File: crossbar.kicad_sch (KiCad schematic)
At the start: 6 parts

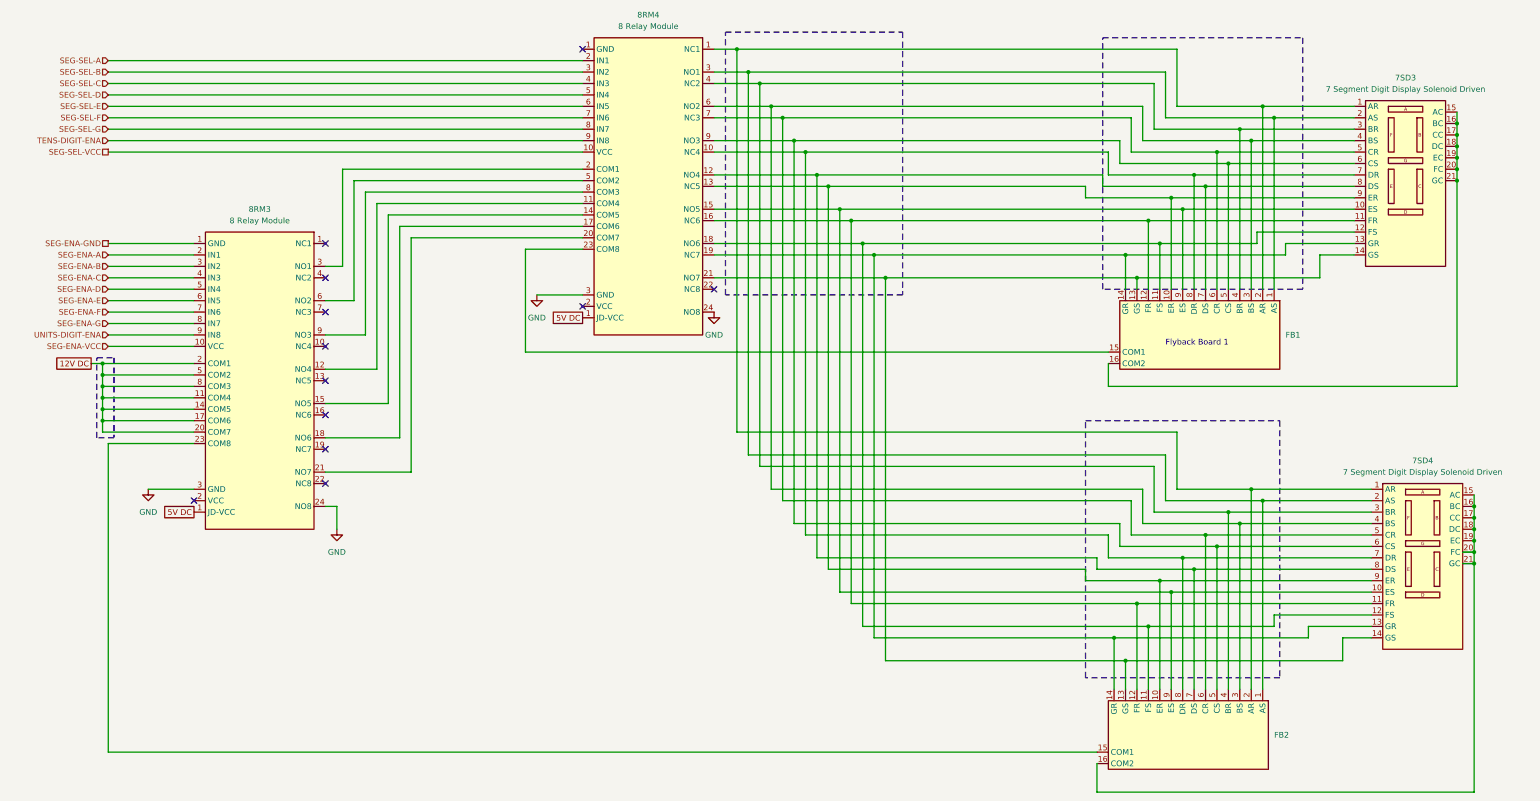
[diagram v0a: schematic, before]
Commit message: lots of diagram changes and software dir.
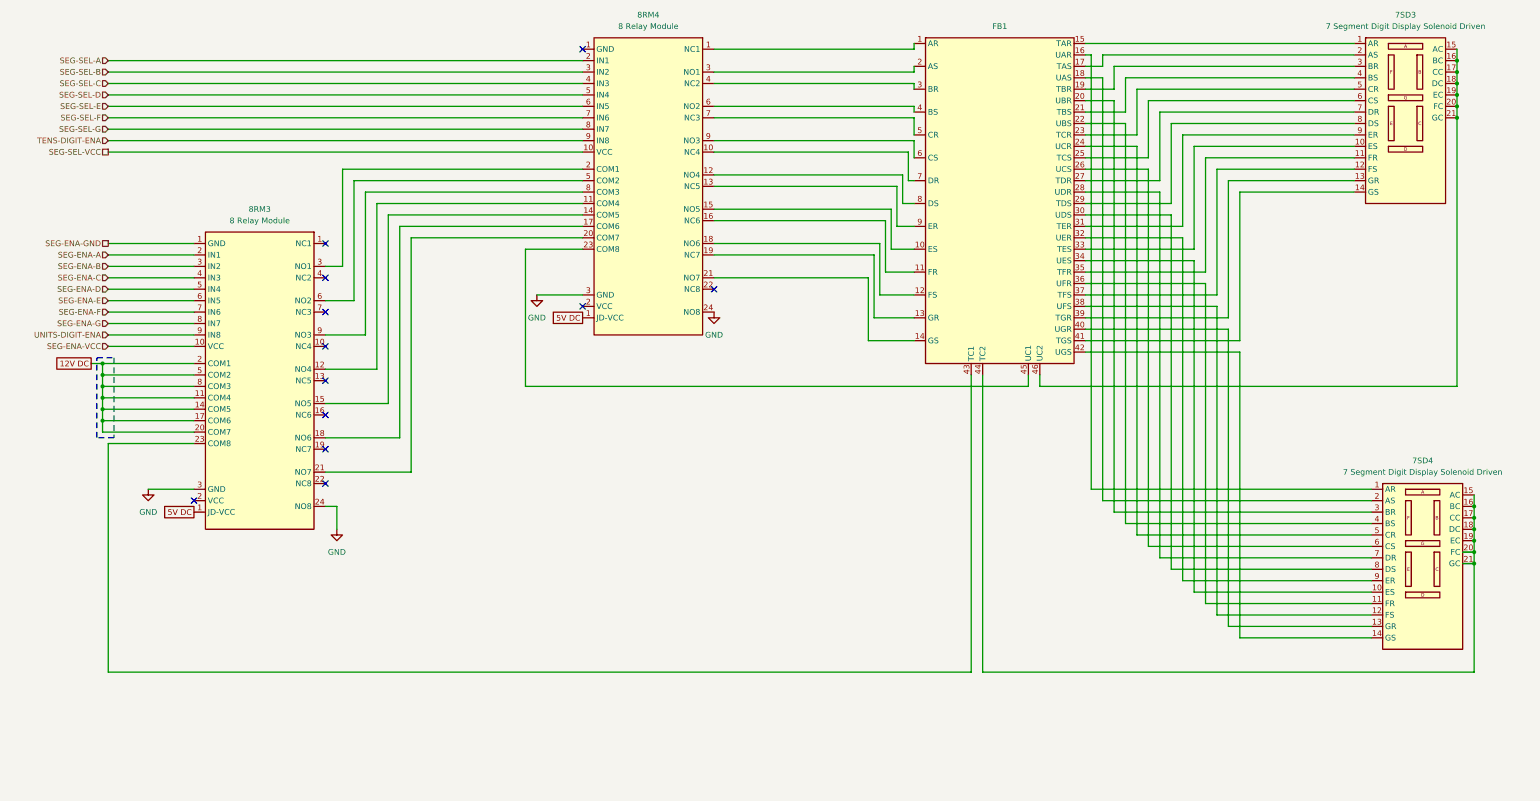
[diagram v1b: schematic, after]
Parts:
- removed FB1, FB2: ~, symbol Project Library:Flyback_Board
- added FB1: ~, symbol Project Library:Flyback_Board_3
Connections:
- net at 8RM4.23 (COM8): now also FB1.45 (UC1)
- net at 7SD3.15 (AC), 7SD3.16 (BC), 7SD3.17 (CC)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: now also FB1.46 (UC2)
- net at 8RM3.23 (COM8): now also FB1.43 (TC1)
- net at 7SD4.15 (AC), 7SD4.16 (BC), 7SD4.17 (CC)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: now also FB1.44 (TC2)
- new net: 8RM3.3 (NO1), 8RM4.2 (VCC)
- new net: 8RM3.6 (NO2), 8RM4.5 (IN4)
- new net: 8RM3.9 (NO3), 8RM4.8 (IN7)
- new net: 8RM4.1 (NC1), FB1.1 (AR)
- new net: 8RM4.10 (VCC), FB1.7 (DR)
- new net: 8RM4.12 (NO4), FB1.8 (DS)
- new net: 8RM4.13 (NC5), FB1.9 (ER)
- new net: 8RM4.15 (NO5), FB1.10 (ES)
- new net: 8RM4.16 (NC6), FB1.11 (FR)
- new net: 8RM4.18 (NO6), FB1.12 (FS)
- new net: 8RM4.19 (NC7), FB1.13 (GR)
- new net: 8RM4.21 (NO7), FB1.14 (GS)
- new net: 8RM4.3 (NO1), FB1.2 (AS)
- new net: 8RM4.4 (NC2), FB1.3 (BR)
- new net: 8RM4.6 (NO2), FB1.4 (BS)
- new net: 8RM4.7 (NC3), FB1.5 (CR)
- new net: 8RM4.9 (NO3), FB1.6 (CS)
- new net: 7SD4.1 (AR), FB1.16 (UAR)
- new net: 7SD4.10 (ES), FB1.34 (UES)
- new net: 7SD4.11 (FR), FB1.36 (UFR)
- new net: 7SD4.12 (FS), FB1.38 (UFS)
- new net: 7SD4.13 (GR), FB1.40 (UGR)
- new net: 7SD4.14 (GS), FB1.42 (UGS)
- new net: 7SD4.2 (AS), FB1.18 (UAS)
- new net: 7SD4.3 (BR), FB1.20 (UBR)
- new net: 7SD4.4 (BS), FB1.22 (UBS)
- new net: 7SD4.5 (CR), FB1.24 (UCR)
- new net: 7SD4.6 (CS), FB1.26 (UCS)
- new net: 7SD4.7 (DR), FB1.28 (UDR)
- new net: 7SD4.8 (DS), FB1.30 (UDS)
- new net: 7SD4.9 (ER), FB1.32 (UER)
- new net: 7SD3.1 (AR), FB1.15 (TAR)
- new net: 7SD3.10 (ES), FB1.33 (TES)
- new net: 7SD3.11 (FR), FB1.35 (TFR)
- new net: 7SD3.12 (FS), FB1.37 (TFS)
- new net: 7SD3.13 (GR), FB1.39 (TGR)
- new net: 7SD3.14 (GS), FB1.41 (TGS)
- new net: 7SD3.2 (AS), FB1.17 (TAS)
- new net: 7SD3.3 (BR), FB1.19 (TBR)
- new net: 7SD3.4 (BS), FB1.21 (TBS)
- new net: 7SD3.5 (CR), FB1.23 (TCR)
- new net: 7SD3.6 (CS), FB1.25 (TCS)
- new net: 7SD3.7 (DR), FB1.27 (TDR)
- new net: 7SD3.8 (DS), FB1.29 (TDS)
- new net: 7SD3.9 (ER), FB1.31 (TER)
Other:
- note removed: "Flyback Board 1"
- moved on the sheet: 7SD3
